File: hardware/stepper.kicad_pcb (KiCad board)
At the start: 4 copper layers, 40 x 40 mm, 125 parts, among them J101 USB-MINI-B-SMD, J102 DRILL, J103 DRILL, J104 DRILL, J105 DRILL, J401 STACK-UP-HIGH, J402 STACK-DOWN, J403 STACK-UP-HIGH, J404 STACK-DOWN, P201 black, P202 green, P301 CON-SENSOR, P302 CON-SENSOR, Q201 AO4438, Q202 AO4421, Q203 2N7002, SW101 Reset, SW102 Erase, U101 AT91SAM3SXB, U102 82400152, U202 TMC2100, U501 LD1117, X101 16Mhz

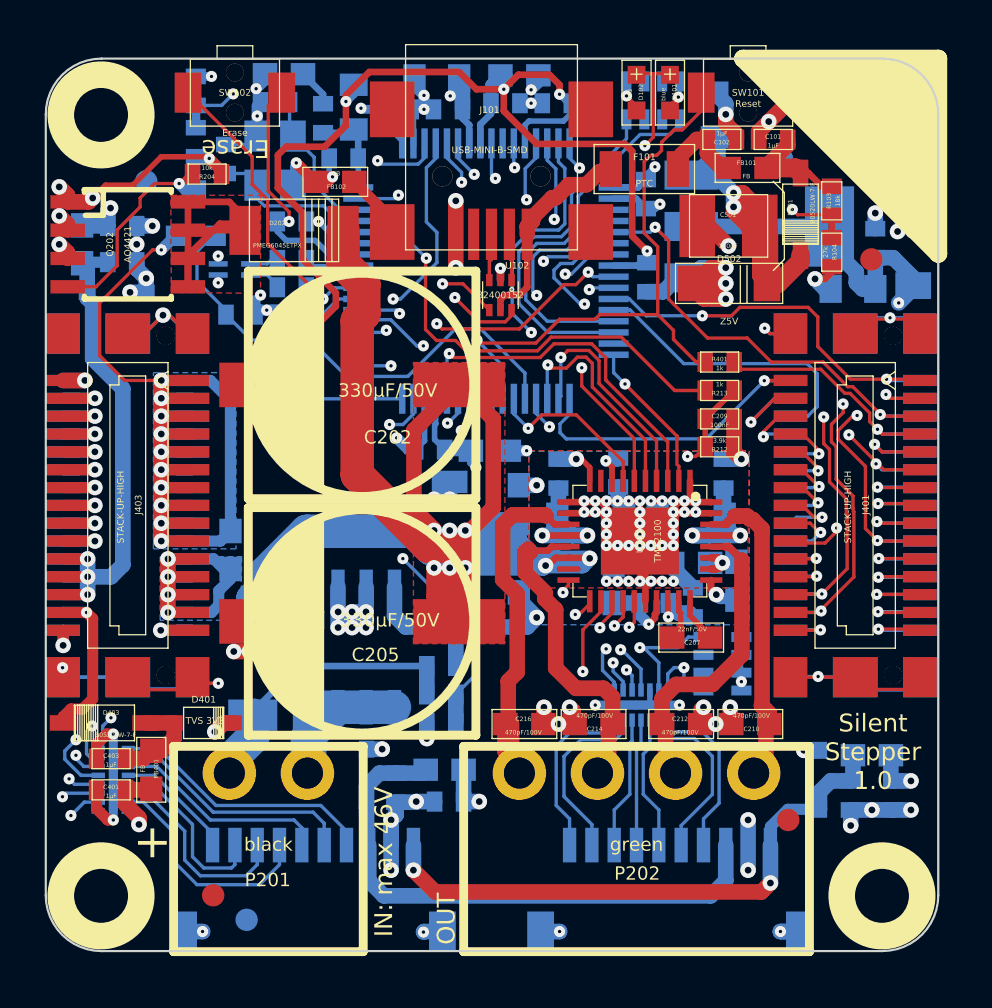
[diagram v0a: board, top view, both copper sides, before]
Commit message: detail routing improvements
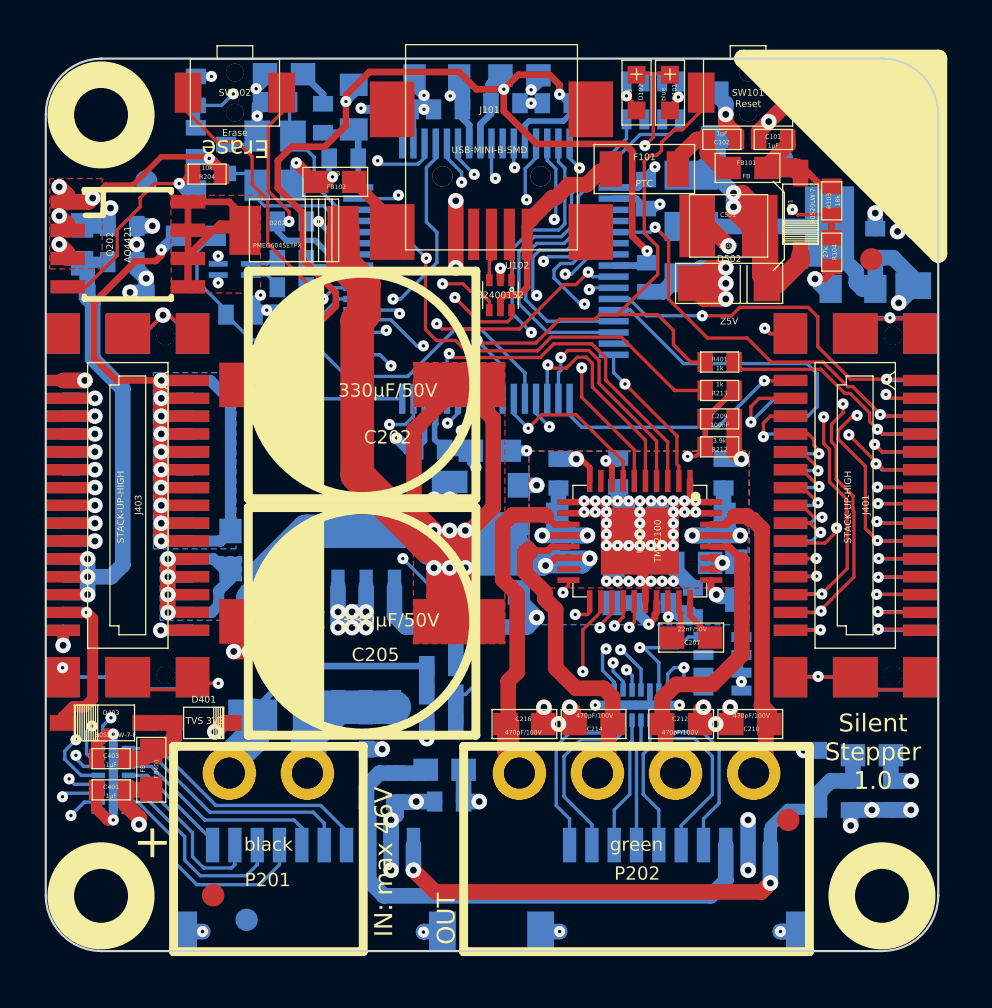
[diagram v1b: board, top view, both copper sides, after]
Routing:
- net STACK-RESET: track 26.7 -> 28.3 mm
- net STACK-I2C-SDA/JTAG-TDI: track 14.4 -> 12.9 mm
- net STACK-I2C-SCL/JTAG-TDO: track 23.3 -> 24.4 mm
- net Net-(J401-Pad6): track 2.99 -> 3.74 mm
- net STACK-PGND: track 218.5 -> 219.2 mm
- net Net-(J401-Pad8): track 3.04 -> 3.73 mm
- net 3V3: track 177.6 -> 178.2 mm
- net Net-(SW102-Pad1): track 13.6 -> 14.1 mm
- net PWR-CFG5: track 24.6 -> 25.1 mm
- added copper zone on F.Cu, net STACK-PVCC
